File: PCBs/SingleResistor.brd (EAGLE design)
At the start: 10.2 x 39.5 mm, 3 parts

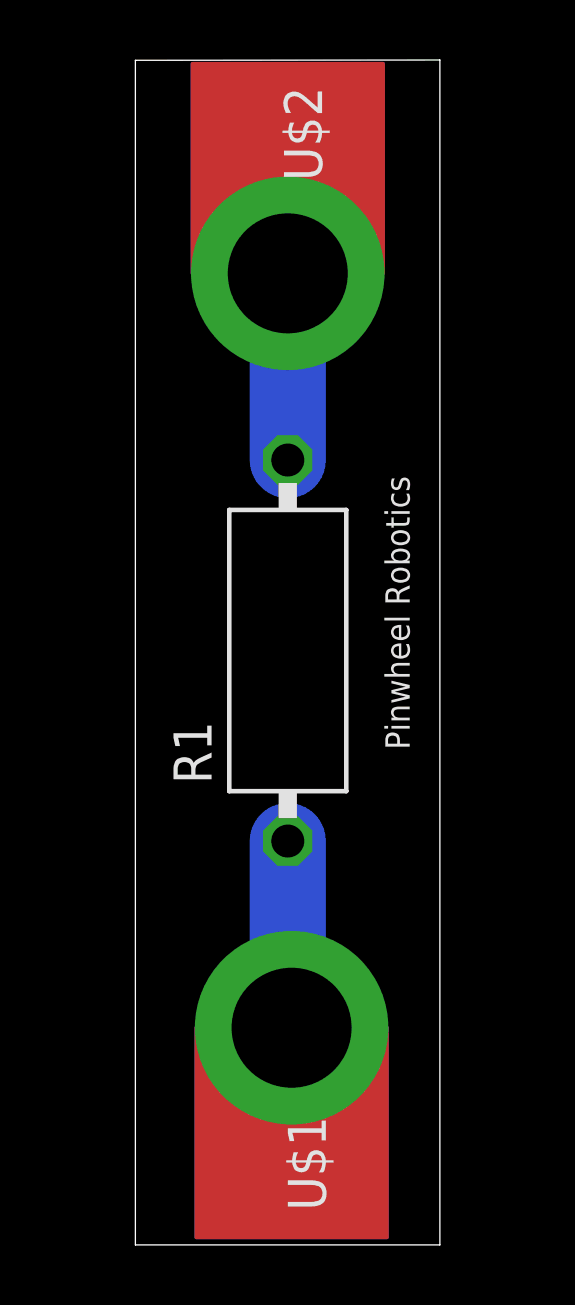
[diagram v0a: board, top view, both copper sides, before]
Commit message: Updated
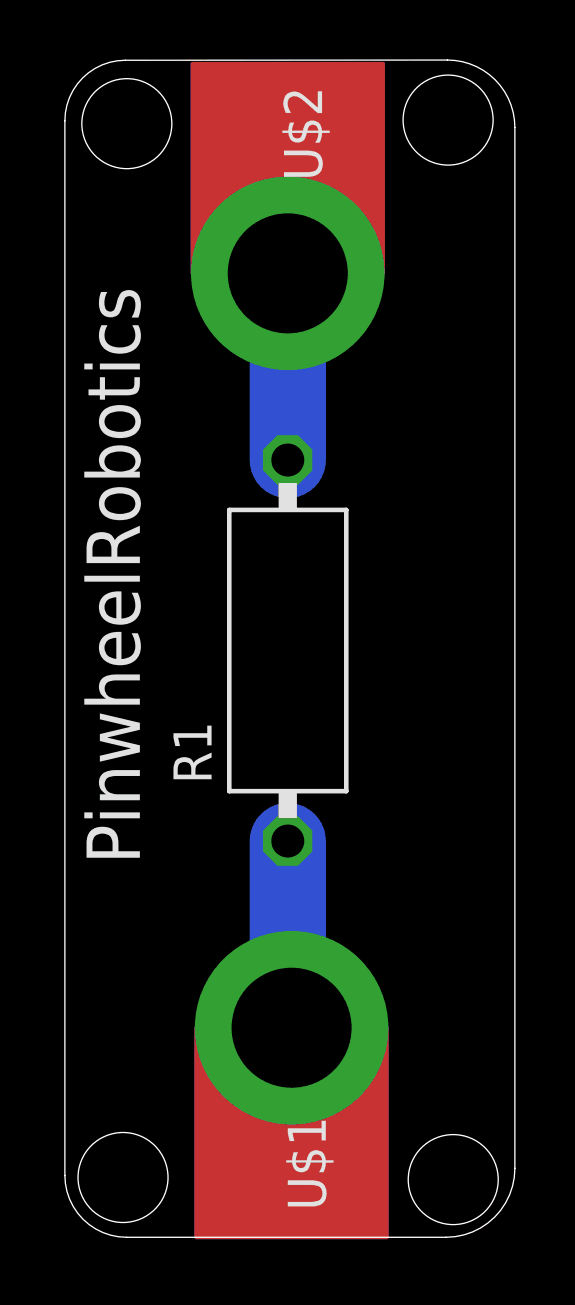
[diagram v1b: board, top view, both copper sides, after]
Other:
- board size 10.2 x 39.5 mm -> 15 x 39.2 mm
- board text added: "PinwheelRobotics"
- board text added: "care@pinwheel.in"
- board text removed: "Pinwheel Robotics"
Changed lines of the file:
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@@
 <setting verticaltext="up"/>
 </settings>
-<grid distance="50" unitdist="mil" unit="mm" style="lines" multiple="1" display="yes" altdistance="5" altunitdist="mil" altunit="mm"/>
+<grid distance="0.5" unitdist="mm" unit="mm" style="lines" multiple="1" display="yes" altdistance="5" altunitdist="mil" altunit="mm"/>
 <layers>
 <layer number="1" name="Top" color="4" fill="1" visible="yes" active="yes"/>
@@
 <layer number="43" name="vRestrict" color="2" fill="10" visible="yes" active="yes"/>
 <layer number="44" name="Drills" color="7" fill="1" visible="no" active="yes"/>
-<layer number="45" name="Holes" color="7" fill="1" visible="no" active="yes"/>
+<layer number="45" name="Holes" color="7" fill="1" visible="yes" active="yes"/>
 <layer number="46" name="Milling" color="3" fill="1" visible="no" active="yes"/>
 <layer number="47" name="Measures" color="7" fill="1" visible="no" active="yes"/>
@@
 <board>
 <plain>
-<wire x1="6.35" y1="3.81" x2="16.5" y2="3.81" width="0" layer="20"/>
-<wire x1="16.5" y1="3.81" x2="16.5" y2="43.307" width="0" layer="20"/>
-<wire x1="16.5" y1="43.307" x2="6.35" y2="43.297" width="0" layer="20"/>
-<wire x1="6.35" y1="43.297" x2="6.35" y2="3.81" width="0" layer="20"/>
-<text x="15.494" y="20.32" size="0.8128" layer="21" rot="R90">Pinwheel Robotics </text>
+<wire x1="4" y1="41.2811875" x2="4" y2="6.123309375" width="0" layer="20"/>
+<wire x1="4" y1="6.123309375" x2="6.059309375" y2="4.064" width="0" layer="20" curve="90"/>
+<wire x1="6.059309375" y1="4.064" x2="16.70208125" y2="4.064" width="0" layer="20"/>
+<wire x1="16.70208125" y1="4.064" x2="19" y2="6.36191875" width="0" layer="20" curve="90"/>
+<wire x1="19" y1="6.36191875" x2="19" y2="41.058371875" width="0" layer="20"/>
+<wire x1="19" y1="41.058371875" x2="16.751375" y2="43.3055" width="0" layer="20" curve="90.038166"/>
+<wire x1="16.751375" y1="43.3055" x2="6.0158125" y2="43.29834375" width="0" layer="20"/>
+<wire x1="6.0158125" y1="43.29834375" x2="4" y2="41.2811875" width="0" layer="20" curve="89.999088"/>
+<hole x="6.065" y="41.185" drill="3"/>
+<hole x="16.774" y="41.304" drill="3"/>
+<hole x="5.938" y="6.057" drill="3"/>
+<hole x="16.945" y="5.987" drill="3"/>
+<text x="6.5" y="16.5" size="1.778" layer="21" rot="R90">PinwheelRobotics</text>
+<text x="17" y="34" size="1.778" layer="22" rot="MR270">care@pinwheel.in</text>
 </plain>
 <attributes>

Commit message: New Update
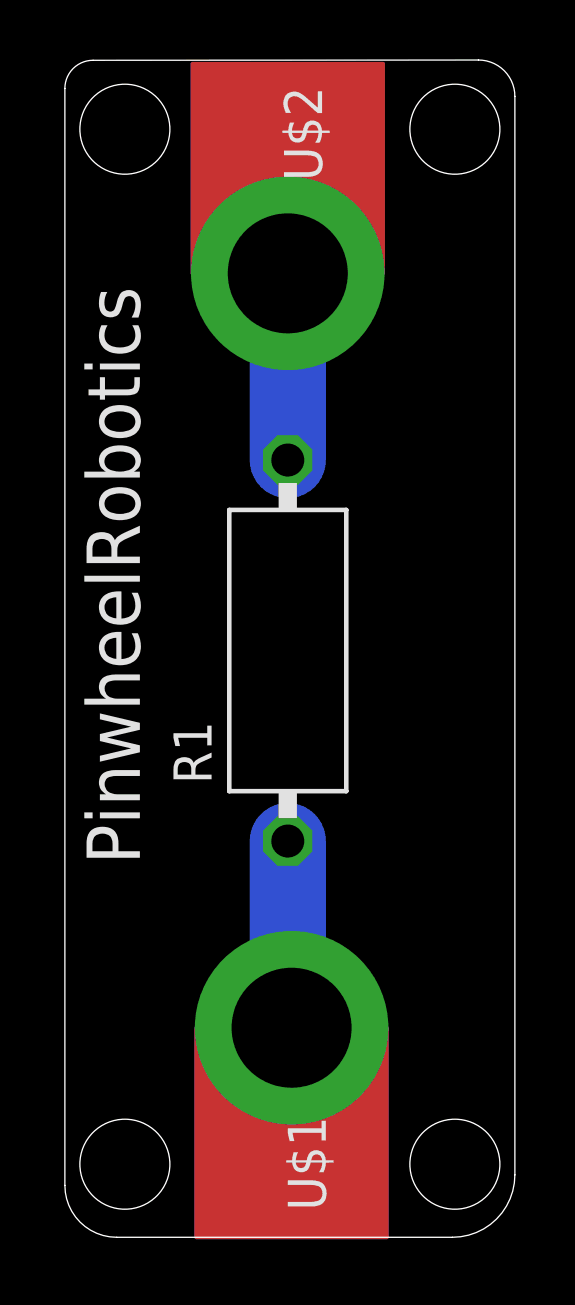
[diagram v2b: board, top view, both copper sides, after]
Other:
- outline, holes or cut-outs redrawn
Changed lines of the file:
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@@
 <board>
 <plain>
-<wire x1="4" y1="41.2811875" x2="4" y2="6.123309375" width="0" layer="20"/>
-<wire x1="4" y1="6.123309375" x2="6.059309375" y2="4.064" width="0" layer="20" curve="90"/>
-<wire x1="6.059309375" y1="4.064" x2="16.70208125" y2="4.064" width="0" layer="20"/>
-<wire x1="16.70208125" y1="4.064" x2="19" y2="6.36191875" width="0" layer="20" curve="90"/>
-<wire x1="19" y1="6.36191875" x2="19" y2="41.058371875" width="0" layer="20"/>
-<wire x1="19" y1="41.058371875" x2="16.751375" y2="43.3055" width="0" layer="20" curve="90.038166"/>
-<wire x1="16.751375" y1="43.3055" x2="6.0158125" y2="43.29834375" width="0" layer="20"/>
-<wire x1="6.0158125" y1="43.29834375" x2="4" y2="41.2811875" width="0" layer="20" curve="89.999088"/>
-<hole x="6.065" y="41.185" drill="3"/>
-<hole x="16.774" y="41.304" drill="3"/>
-<hole x="5.938" y="6.057" drill="3"/>
-<hole x="16.945" y="5.987" drill="3"/>
+<wire x1="4" y1="42.358221875" x2="4" y2="5.791765625" width="0" layer="20"/>
+<wire x1="4" y1="5.791765625" x2="5.727765625" y2="4.064" width="0" layer="20" curve="90"/>
+<wire x1="5.727765625" y1="4.064" x2="16.91804375" y2="4.064" width="0" layer="20"/>
+<wire x1="16.91804375" y1="4.064" x2="19" y2="6.14595625" width="0" layer="20" curve="90"/>
+<wire x1="19" y1="6.14595625" x2="19" y2="42.09330625" width="0" layer="20"/>
+<wire x1="19" y1="42.09330625" x2="17.78630625" y2="43.306190625" width="0" layer="20" curve="90.038234"/>
+<wire x1="17.78630625" y1="43.306190625" x2="4.938778125" y2="43.297625" width="0" layer="20"/>
+<wire x1="4.938778125" y1="43.297625" x2="4" y2="42.358221875" width="0" layer="20" curve="90.077877"/>
+<hole x="6" y="41" drill="3"/>
+<hole x="17" y="41" drill="3"/>
+<hole x="6" y="6.5" drill="3"/>
+<hole x="17" y="6.5" drill="3"/>
 <text x="6.5" y="16.5" size="1.778" layer="21" rot="R90">PinwheelRobotics</text>
 <text x="17" y="34" size="1.778" layer="22" rot="MR270">care@pinwheel.in</text>
